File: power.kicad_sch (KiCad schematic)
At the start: 10 parts, among them J1 USB4215-03-A, U2 NCP1117 3.3, U4 USBLC6-2SC6

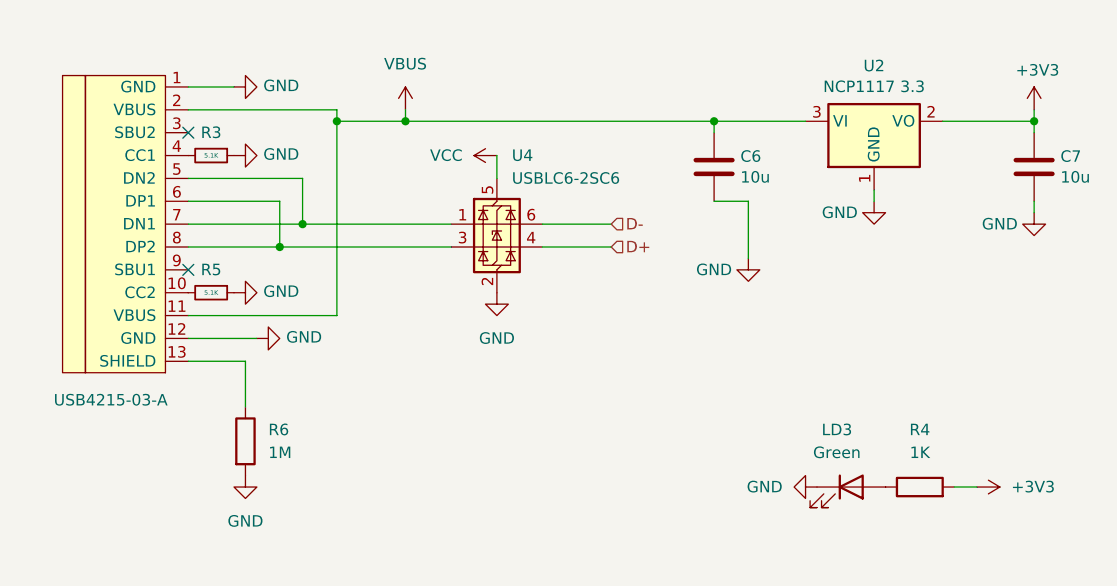
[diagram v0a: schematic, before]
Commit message: Work-in-progress
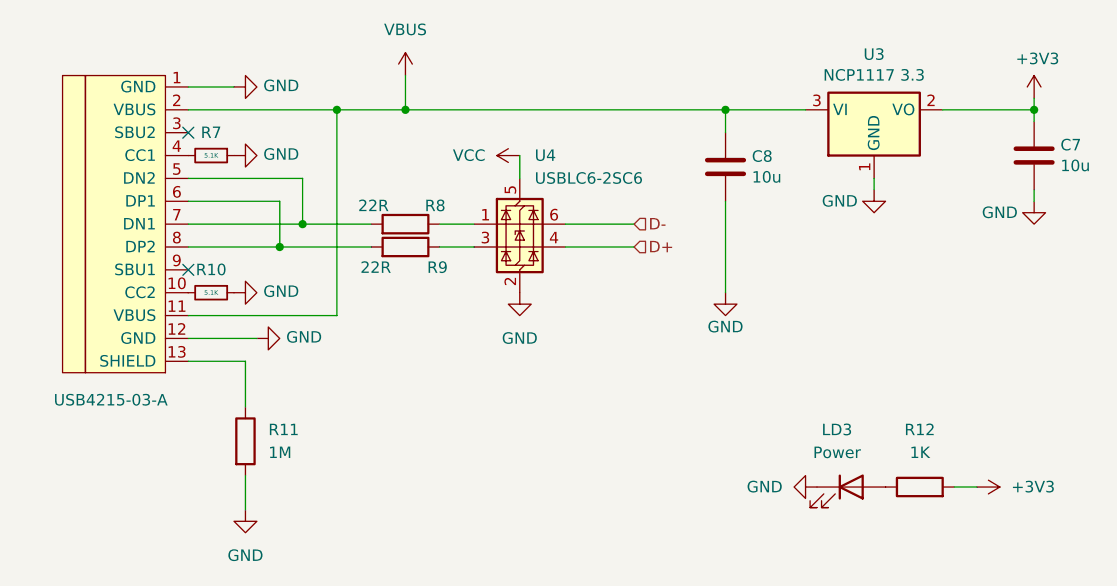
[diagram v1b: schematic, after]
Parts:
- added R8, R9: 22R, FRANK:Resistor (0805), symbol Device:R
- C7: LCSC C1713 -> (none)
- C8: renamed from C6; LCSC C1713 -> (none)
- J2: renamed from J1; LCSC C165948 -> (none)
- LD3: value Green -> Power
- R10: renamed from R5; LCSC C3152211 -> (none)
- R11: renamed from R6; LCSC C3152182 -> (none)
- R12: renamed from R4; LCSC C17513 -> (none)
- R7: renamed from R3; LCSC C3152211 -> (none)
- U3: renamed from U2; LCSC C5346136 -> (none)
- U4: footprint Package_TO_SOT_SMD:SOT-23-6 -> FRANK:SOT-23-6
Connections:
- net at J2.5 (DN2), J2.7 (DN1): now also R8.2; no longer U4.1 (I/O1)
- net at J2.6 (DP1), J2.8 (DP2): now also R9.2; no longer U4.3 (I/O2)
- new net: R8.1, U4.1 (I/O1)
- new net: R9.1, U4.3 (I/O2)
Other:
- moved on the sheet: C7, C8, U3, U4
